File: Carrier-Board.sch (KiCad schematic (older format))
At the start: 45 parts, among them J1 CONN_3-6318491-6, J10 Conn_02x03_Odd_Even, J2 Conn_01x0, J3 Conn_02x26_Odd_Even, J4 SI-51009-F, J5 Conn_02x26_Odd_Even, J6 Conn_01x03_Male, J7 Conn_01x03_Male, J8 Conn_01x06_Male, J9 Conn_02x04_Odd_Even, SW1 SW_Push, SW2 SW_Push, SW3 SW_Push, U1 MPM3620, U2 MPM3620, U9 MSATA-Socket

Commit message: asdf
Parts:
- removed C1, C3: 10uF, Capacitors_SMD:C_0805, symbol CP
- removed C2, C4: 22uF, Capacitors_SMD:C_0805, symbol CP
- removed D5: D_Zener 9V, Diodes_SMD:D_SOD-323, symbol D_Zener
- removed D6, D7, D8: LED, Diodes_SMD:D_1206, symbol LED
- removed J10: Conn_02x03_Odd_Even, Pin_Headers:Pin_Header_Angled_2x03_Pitch2.54mm, symbol Conn_02x03_Odd_Even
- removed J2: Conn_01x0, Connectors:Barrel_Jack_CUI_PJ-036AH-SMT, symbol Barrel_Jack
- removed J4: SI-51009-F, Carrier-Board:SI-51009-F, symbol Conn_02x09_Odd_Even
- removed J6, J7: Conn_01x03_Male, Pin_Headers:Pin_Header_Angled_1x03_Pitch2.54mm, symbol Conn_01x03_Male
- removed J8: Conn_01x06_Male, Pin_Headers:Pin_Header_Angled_1x06_Pitch2.54mm, symbol Conn_01x06_Male
- removed J9: Conn_02x04_Odd_Even, Pin_Headers:Pin_Header_Angled_2x04_Pitch2.54mm, symbol Conn_02x04_Odd_Even
- removed R1, R5: 160k, Resistors_SMD:R_0805, symbol R
- removed R10, R9: 330, Resistors_SMD:R_0805, symbol R
- removed R11, R12, R13: 10K, Resistors_SMD:R_0603, symbol R
- removed R2: 30.1k, Resistors_SMD:R_0805, symbol R
- removed R23: 330, Resistors_SMD:R_0603, symbol R
- removed R24: 180, Resistors_SMD:R_0603, symbol R
- removed R25: 1k, Resistors_SMD:R_0603, symbol R
- removed R3, R7: 100k, Resistors_SMD:R_0805, symbol R
- removed R4: 63.4k, Resistors_SMD:R_0805, symbol R
- removed R6: 51k, Resistors_SMD:R_0805, symbol R
- removed R8: 56k, Resistors_SMD:R_0805, symbol R
- removed SW1, SW2, SW3: SW_Push, Buttons_Switches_SMD:SW_SPST_B3U-1000P, symbol SW_Push
- removed U1, U2: MPM3620, BusSimulator:QFN-20, symbol MPM3620
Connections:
- net labels removed: +12V, +5V, GNDA, PCE3895CT-ND, PCE3900CT-ND, SPI_POWER
- wire segments 102 -> 24
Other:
- note removed: "12V\n"
- note removed: "3V3\n"
- note removed: "5V SBY\n"
- note removed: "Break out\n"
- note removed: "Ethernet"
- note removed: "GPIO\n"
- note removed: "I2C\n"
- note removed: "LED Indicators\n"
- note removed: "MISC SHIT"
- note removed: "Rs232\n"
- note removed: "SPI\n"
- note removed: "Voltage Supply"

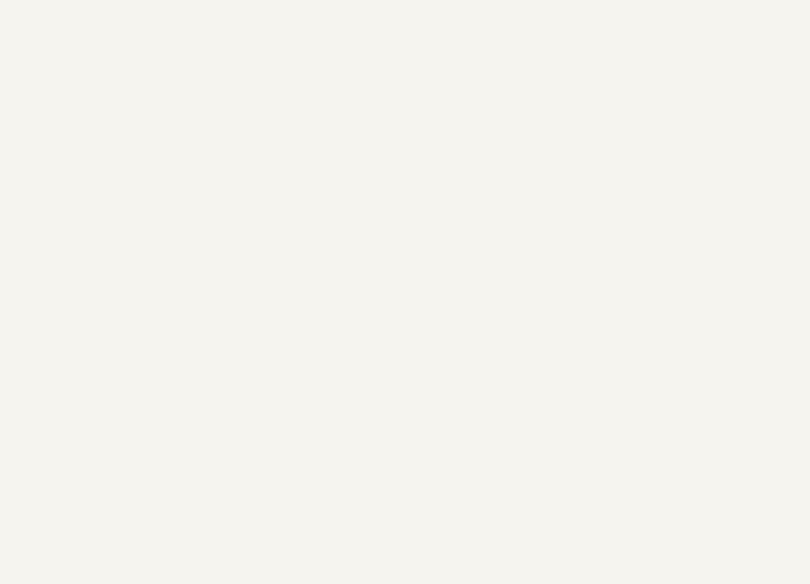
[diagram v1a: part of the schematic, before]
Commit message: stuff
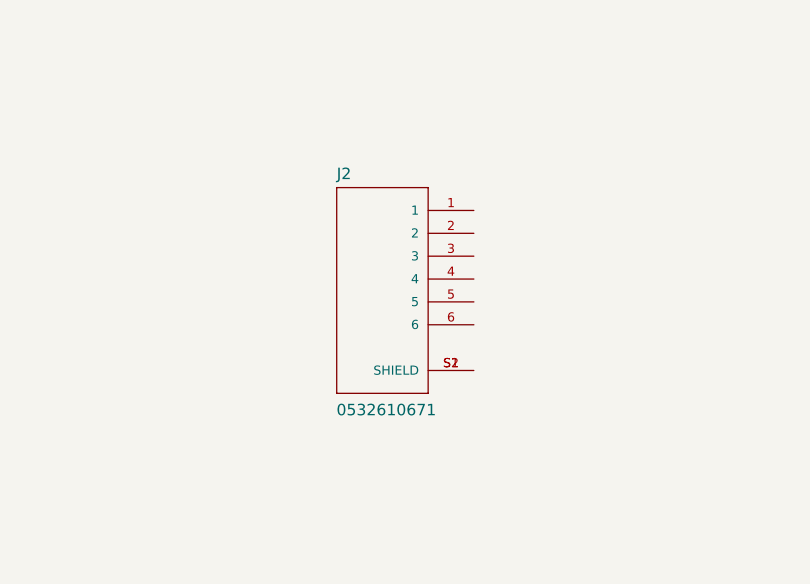
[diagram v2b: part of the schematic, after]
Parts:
- added J2: 0532610671, MOLEX_0532610671, symbol 0532610671
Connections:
- new net: J2.S1 (SHIELD), J2.S2 (SHIELD)
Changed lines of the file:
@@
 LIBS:Carrier-Board
 LIBS:SI-51009-F
+LIBS:0532610271
+LIBS:0532610371
+LIBS:0532610471
+LIBS:0532610671
 LIBS:Carrier-Board-cache
 EELAYER 25 0
@@
 +3.3V
 $Comp
-L GNDREF #PWR022
+L GNDREF #PWR8
 U 1 1 5A0C1B77
 P 3700 8250
-F 0 "#PWR022" H 3700 8000 50  0001 C CNN
+F 0 "#PWR8" H 3700 8000 50  0001 C CNN
 F 1 "GNDREF" H 3700 8100 50  0000 C CNN
 F 2 "" H 3700 8250 50  0001 C CNN
@@
 $EndComp
 $Comp
-L GNDREF #PWR023
+L GNDREF #PWR9
 U 1 1 5A0C1C29
 P 3900 10650
-F 0 "#PWR023" H 3900 10400 50  0001 C CNN
+F 0 "#PWR9" H 3900 10400 50  0001 C CNN
 F 1 "GNDREF" H 3900 10500 50  0000 C CNN
 F 2 "" H 3900 10650 50  0001 C CNN
@@
 $EndComp
 $Comp
-L GNDREF #PWR024
+L GNDREF #PWR12
 U 1 1 5A0C1CDB
 P 4000 9450
-F 0 "#PWR024" H 4000 9200 50  0001 C CNN
+F 0 "#PWR12" H 4000 9200 50  0001 C CNN
 F 1 "GNDREF" H 4000 9300 50  0000 C CNN
 F 2 "" H 4000 9450 50  0001 C CNN
@@
 $EndComp
 $Comp
-L GNDREF #PWR025
+L GNDREF #PWR11
 U 1 1 5A0C1D8D
 P 4000 9050
-F 0 "#PWR025" H 4000 8800 50  0001 C CNN
+F 0 "#PWR11" H 4000 8800 50  0001 C CNN
 F 1 "GNDREF" H 4000 8900 50  0000 C CNN
 F 2 "" H 4000 9050 50  0001 C CNN
@@
 $EndComp
 $Comp
-L GNDREF #PWR026
+L GNDREF #PWR10
 U 1 1 5A0C1E3F
 P 4000 8750
-F 0 "#PWR026" H 4000 8500 50  0001 C CNN
+F 0 "#PWR10" H 4000 8500 50  0001 C CNN
 F 1 "GNDREF" H 4000 8600 50  0000 C CNN
 F 2 "" H 4000 8750 50  0001 C CNN
@@
 $EndComp
 $Comp
-L GNDREF #PWR027
+L GNDREF #PWR13
 U 1 1 5A0C1EF1
 P 4000 9850
-F 0 "#PWR027" H 4000 9600 50  0001 C CNN
+F 0 "#PWR13" H 4000 9600 50  0001 C CNN
 F 1 "GNDREF" H 4000 9700 50  0000 C CNN
 F 2 "" H 4000 9850 50  0001 C CNN
@@
 SATA0_RX-
 $Comp
-L GNDREF #PWR028
+L GNDREF #PWR6
 U 1 1 5A0C49FB
 P 1800 10400
-F 0 "#PWR028" H 1800 10150 50  0001 C CNN
+F 0 "#PWR6" H 1800 10150 50  0001 C CNN
 F 1 "GNDREF" H 1800 10250 50  0000 C CNN
 F 2 "" H 1800 10400 50  0001 C CNN
@@
 $EndComp
 $Comp
-L GNDREF #PWR029
+L GNDREF #PWR7
 U 1 1 5A0C4BAB
 P 1900 10050
-F 0 "#PWR029" H 1900 9800 50  0001 C CNN
+F 0 "#PWR7" H 1900 9800 50  0001 C CNN
 F 1 "GNDREF" H 1900 9900 50  0000 C CNN
 F 2 "" H 1900 10050 50  0001 C CNN
@@
 Sata Connector\n
 $Comp
-L GNDREF #PWR030
+L GNDREF #PWR3
 U 1 1 5A0C6A3D
 P 1450 8950
-F 0 "#PWR030" H 1450 8700 50  0001 C CNN
+F 0 "#PWR3" H 1450 8700 50  0001 C CNN
 F 1 "GNDREF" H 1450 8800 50  0000 C CNN
 F 2 "" H 1450 8950 50  0001 C CNN
@@
 $EndComp
 $Comp
-L GNDREF #PWR031
+L GNDREF #PWR4
 U 1 1 5A0C6D48
 P 1500 9350
-F 0 "#PWR031" H 1500 9100 50  0001 C CNN
+F 0 "#PWR4" H 1500 9100 50  0001 C CNN
 F 1 "GNDREF" H 1500 9200 50  0000 C CNN
 F 2 "" H 1500 9350 50  0001 C CNN
@@
 $EndComp
 $Comp
-L GNDREF #PWR032
+L GNDREF #PWR5
 U 1 1 5A0C77C7
 P 1600 8450
-F 0 "#PWR032" H 1600 8200 50  0001 C CNN
+F 0 "#PWR5" H 1600 8200 50  0001 C CNN
 F 1 "GNDREF" H 1600 8300 50  0000 C CNN
 F 2 "" H 1600 8450 50  0001 C CNN
@@
 $EndComp
 $Comp
-L GNDREF #PWR033
+L GNDREF #PWR1
 U 1 1 5A0DCFAA
 P 750 8350
-F 0 "#PWR033" H 750 8100 50  0001 C CNN
+F 0 "#PWR1" H 750 8100 50  0001 C CNN
 F 1 "GNDREF" H 750 8200 50  0000 C CNN
 F 2 "" H 750 8350 50  0001 C CNN
@@
 $EndComp
 $Comp
-L GNDREF #PWR034
+L GNDREF #PWR2
 U 1 1 5A0DD07C
 P 1100 9050
-F 0 "#PWR034" H 1100 8800 50  0001 C CNN
+F 0 "#PWR2" H 1100 8800 50  0001 C CNN
 F 1 "GNDREF" H 1100 8900 50  0000 C CNN
 F 2 "" H 1100 9050 50  0001 C CNN
@@
 $EndComp
 $Comp
-L GNDREF #PWR035
+L GNDREF #PWR14
 U 1 1 5A0DDC34
 P 4500 8450
-F 0 "#PWR035" H 4500 8200 50  0001 C CNN
+F 0 "#PWR14" H 4500 8200 50  0001 C CNN
 F 1 "GNDREF" H 4500 8300 50  0000 C CNN
 F 2 "" H 4500 8450 50  0001 C CNN
@@
 Wire Bus Line
 	16100 3900 4700 3900
+$Comp
+L 0532610671 J2
+U 1 1 5AB9DE55
+P 2450 1900
+F 0 "J2" H 2250 2331 50  0000 L BNN
+F 1 "0532610671" H 2249 1298 50  0000 L BNN
+F 2 "MOLEX_0532610671" H 2450 1900 50  0001 L BNN
+F 3 "None" H 2450 1900 50  0001 L BNN
+F 4 "Good" H 2450 1900 50  0001 L BNN "Field4"
+F 5 "0532610671" H 2450 1900 50  0001 L BNN "Field5"
+F 6 "1.25mm (.049) Pitch PicoBlade Header, Surface Mount, Right Angle, Lead-free, 6 Circuits" H 2450 1900 50  0001 L BNN "Field6"
+F 7 "0.82 USD" H 2450 1900 50  0001 L BNN "Field7"
+F 8 "Molex" H 2450 1900 50  0001 L BNN "Field8"
+	1    2450 1900
+	1    0    0    -1
+$EndComp
 $EndSCHEMATC
